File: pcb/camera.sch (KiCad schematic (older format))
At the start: 58 parts, among them P10 OUTP, P4 HORI, P5 OUTP, P6 POWER, P7 VERT, Q1 2SC5095, Q2 MT3S20TU, Q3 2SC5095, Q4 MT3S20TU, U10 ICX825AQA, U4 TXB0104, U5 ADDI9023, U6 ADA4800, U9 ADA4800

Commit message: ready for ordering
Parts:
- Q1, Q2, Q3, Q4: symbol Q_NPN_BEC -> Q_NPN_BCE
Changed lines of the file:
@@
 $EndComp
 $Comp
-L Q_NPN_BEC Q1
+L Q_NPN_BCE Q1
 U 1 1 5590D88C
 P 7450 5150
@@
 $EndComp
 $Comp
-L Q_NPN_BEC Q2
+L Q_NPN_BCE Q2
 U 1 1 5590DA54
 P 7900 4800
@@
 $EndComp
 $Comp
-L Q_NPN_BEC Q3
+L Q_NPN_BCE Q3
 U 1 1 5590FE91
 P 9550 5150
@@
 $EndComp
 $Comp
-L Q_NPN_BEC Q4
+L Q_NPN_BCE Q4
 U 1 1 5590FF55
 P 10000 4800

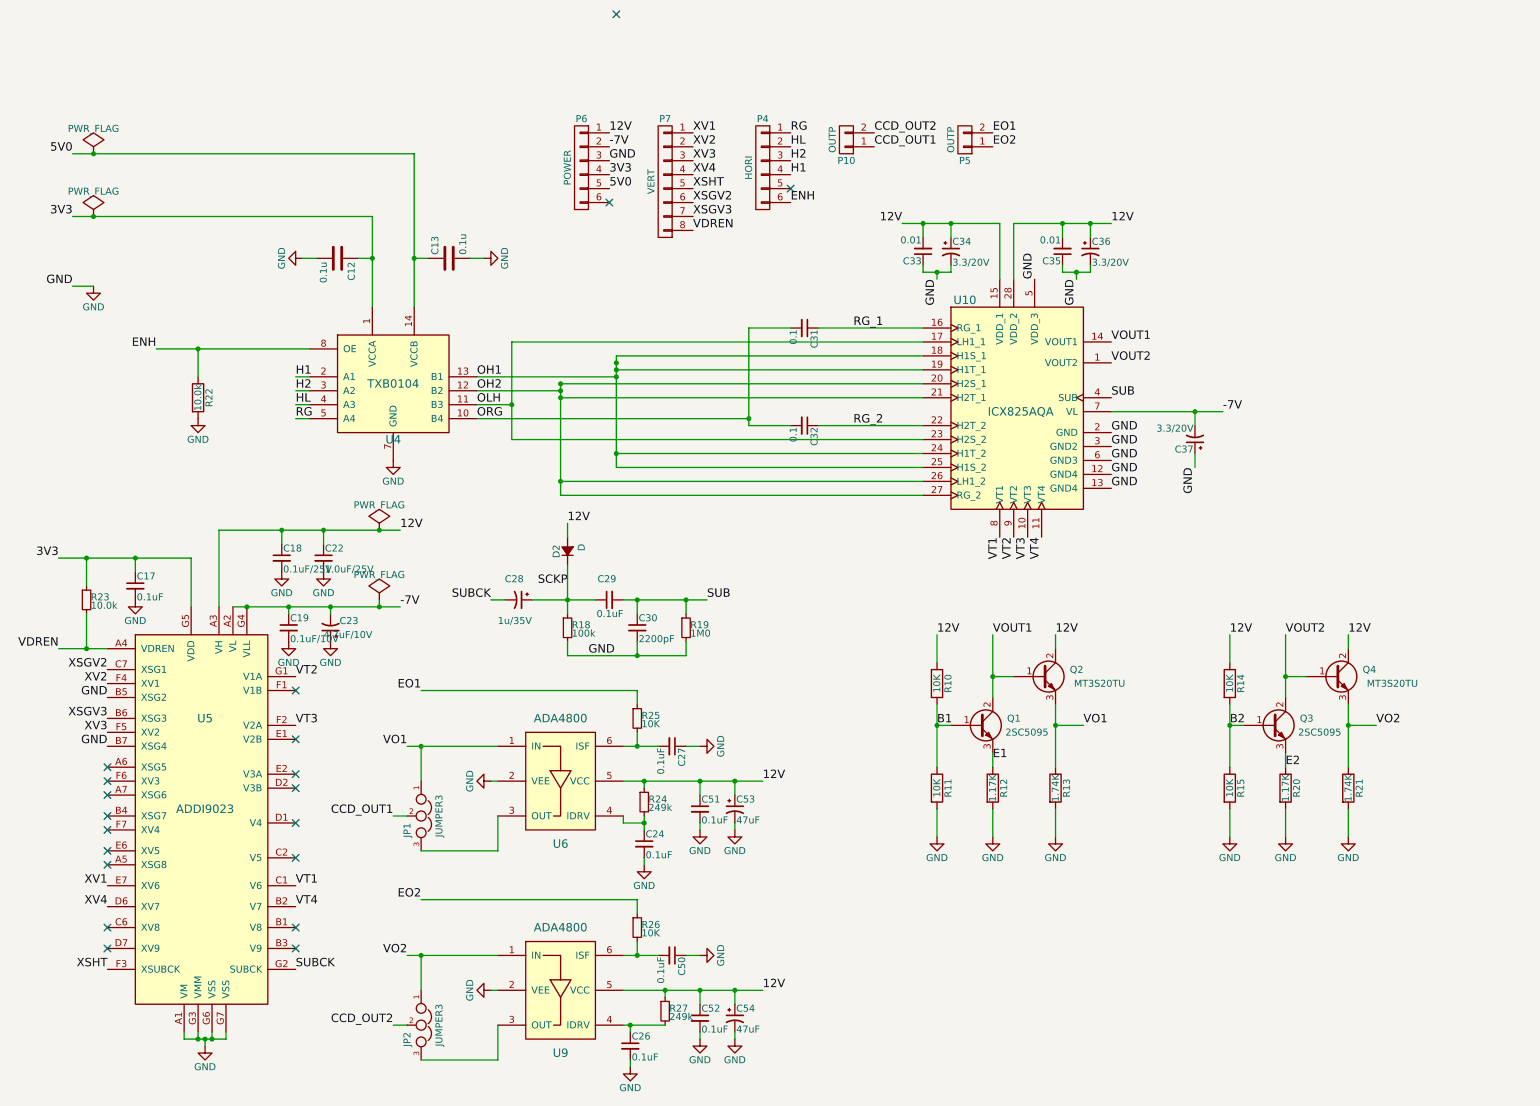
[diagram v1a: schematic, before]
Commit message: Latest, greatest.
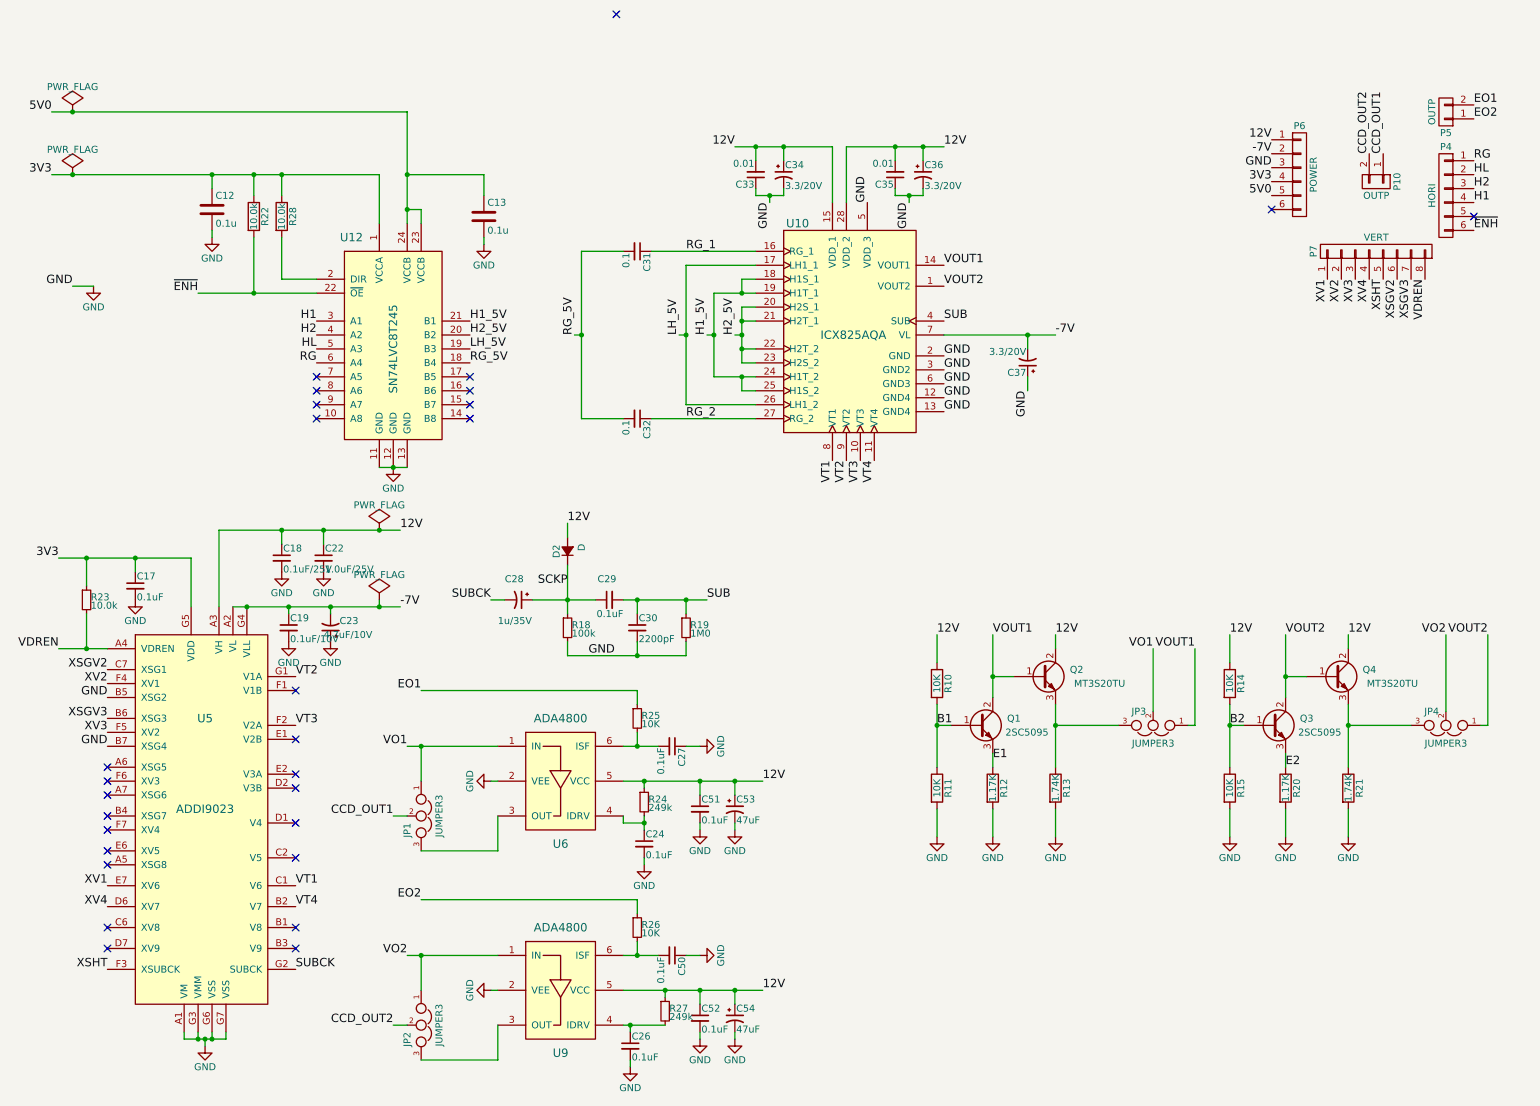
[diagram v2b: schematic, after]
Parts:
- removed U4: TXB0104, Housings_SSOP:TSSOP-14_4.4x5mm_Pitch0.65mm, symbol TXB0104
- added JP3, JP4: JUMPER3, xess:xess-JP2, symbol JUMPER3
- added R28: 10.0k, Resistors_SMD:R_0603_HandSoldering, symbol R
- added U12: SN74LVC8T245, Housings_SSOP:TSSOP-24_4.4x7.8mm_Pitch0.65mm, symbol SN74LVC8T245
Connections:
- net 3V3: now also R22.1, R28.1, U12.1 (VCCA)
- net 5V0: now also U12.23 (VCCB), U12.24 (VCCB)
- net GND: now also U12.11 (GND), U12.12 (GND), U12.13 (GND); no longer R22.2
- net H1: now also U12.3 (A1)
- net H2: now also U12.4 (A2)
- net HL: now also U12.5 (A3)
- net RG: now also U12.6 (A4)
- net RG_2: now also U10.27 (RG_2); no longer U10.22 (H2T_2)
- net VO1: now also JP3.2; no longer Q2.3 (E), R13.1
- net VO2: now also JP4.2; no longer Q4.3 (E), R21.1
- net VOUT1: now also JP3.1
- net VOUT2: now also JP4.1
- net ENH renamed ~ENH~
- net ~ENH~: now also R22.2, U12.22 (~OE); no longer R22.1
- net OH1 renamed H1_5V
- net H1_5V: now also U12.21 (B1)
- net OH2 renamed H2_5V
- net H2_5V: now also U10.22 (H2T_2), U10.23 (H2S_2), U12.20 (B2); no longer U10.26 (LH1_2), U10.27 (RG_2)
- net OLH renamed LH_5V
- net LH_5V: now also U10.26 (LH1_2), U12.19 (B3); no longer U10.23 (H2S_2)
- net ORG renamed RG_5V
- net RG_5V: now also U12.18 (B4)
- new net: JP3.3, Q2.3 (E), R13.1
- new net: JP4.3, Q4.3 (E), R21.1
- new net: R28.2, U12.2 (DIR)
- no-connect marks 20 -> 28
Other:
- moved on the sheet: C12, C13, C31, C32, C33, C34, C35, C36, C37, P10, P4, P5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

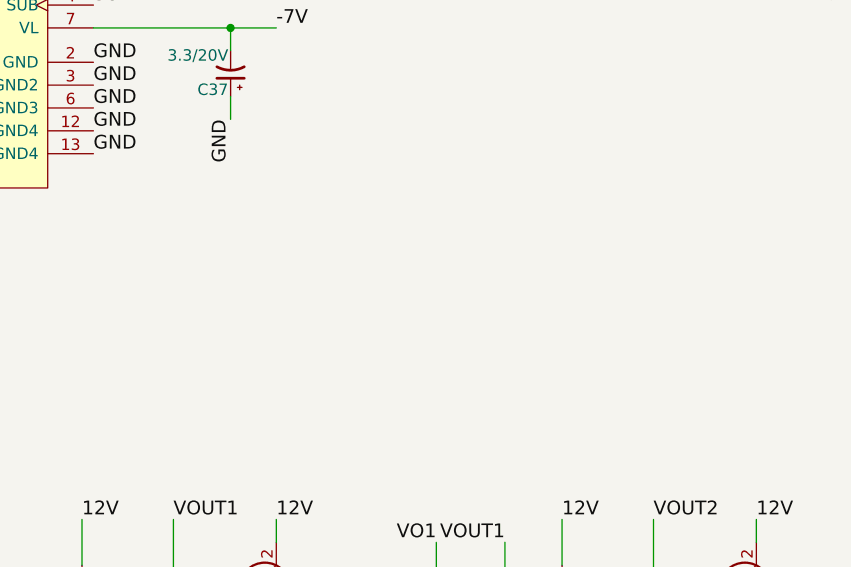
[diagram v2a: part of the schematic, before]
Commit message: latest
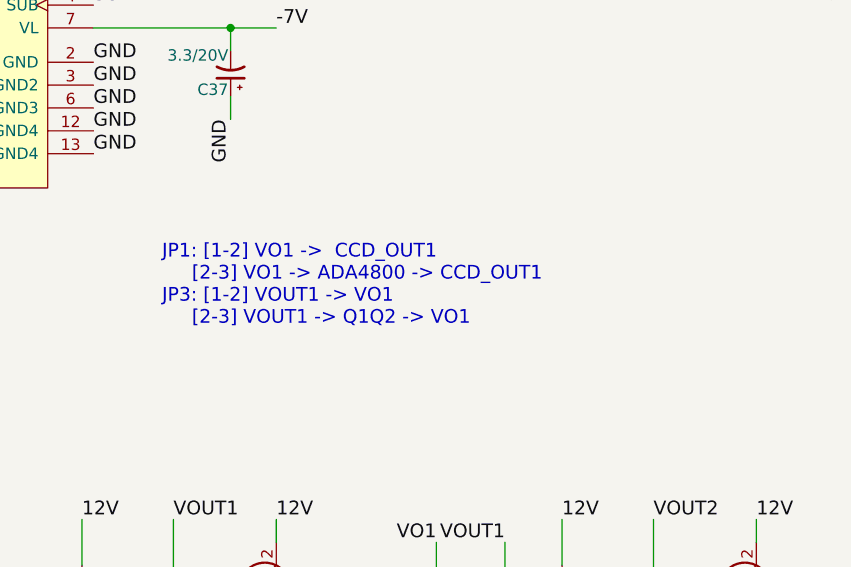
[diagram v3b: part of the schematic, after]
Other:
- note added: "JP1: [1-2] VO1 -> CCD_OUT1\n [2-3] VO1 -> ADA4800 -> CCD_OUT1\nJP3: [1-2] VOUT1 -> VO1\n [2-3] VOUT1 -> Q1Q2 -> VO1\n\n\n"
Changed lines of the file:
@@
 Text Label 5700 2350 1    60   ~ 0
 H2_5V
+Text Notes 7500 3850 0    60   ~ 0
+JP1: [1-2] VO1 ->  CCD_OUT1\n     [2-3] VO1 -> ADA4800 -> CCD_OUT1\nJP3: [1-2] VOUT1 -> VO1\n     [2-3] VOUT1 -> Q1Q2 -> VO1\n\n\n
 $EndSCHEMATC
